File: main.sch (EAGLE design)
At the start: 45 parts, among them IC1 ATTINY13A-SSH, IC2 TP4056-42-ESOP8, IC3 LM27313XMFX_NOPB, IC4 TPL5110DDCT, IC5 ATTINY13A-SSH, T1A 2N4401, T1B NPN, X1 MINI-USB-UX60A-MB-5ST, X2 332-02

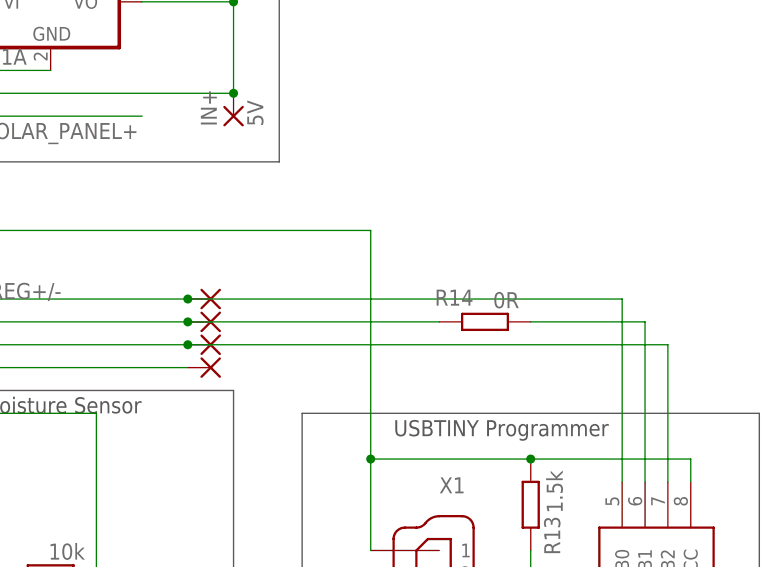
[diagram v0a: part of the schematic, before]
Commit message: updates
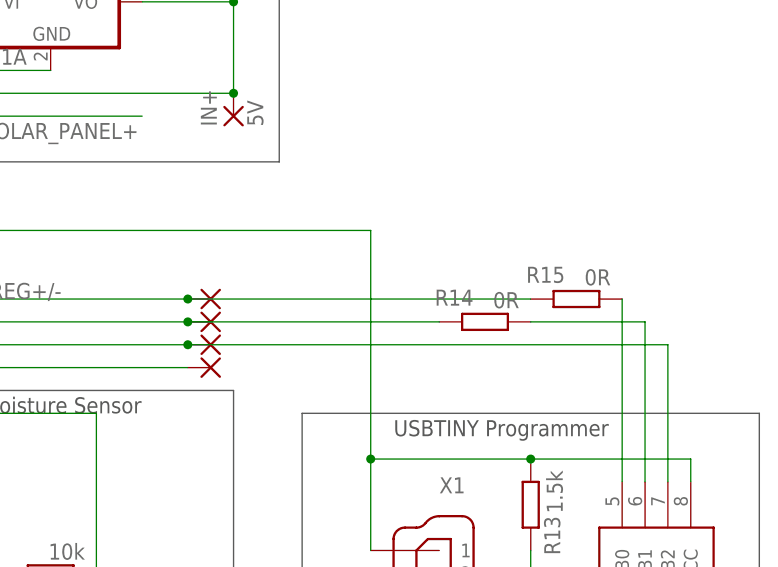
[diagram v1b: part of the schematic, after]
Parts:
- added R15: 0R, resistor:R-EU_R0402
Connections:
- new net N$16: IC5.PB0, R15.1
- net SOLAR_REG+/-: now also R15.2; no longer IC5.PB0
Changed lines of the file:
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@@
 <?xml version="1.0" encoding="utf-8"?>
 <!DOCTYPE eagle SYSTEM "eagle.dtd">
-<eagle version="9.5.2">
+<eagle version="9.6.0">
 <drawing>
 <settings>
@@
 <part name="GND4" library="supply1" library_urn="urn:adsk.eagle:library:371" deviceset="GND" device=""/>
 <part name="R14" library="resistor" library_urn="urn:adsk.eagle:library:348" deviceset="R-EU_" device="R0402" package3d_urn="urn:adsk.eagle:package:26058/1" value="0R"/>
+<part name="R15" library="resistor" library_urn="urn:adsk.eagle:library:348" deviceset="R-EU_" device="R0402" package3d_urn="urn:adsk.eagle:package:26058/1" value="0R"/>
 </parts>
 <sheets>
@@
 <attribute name="VALUE" x="163.83" y="59.182" size="1.778" layer="96" rot="R180"/>
 </instance>
+<instance part="R15" gate="G$1" x="170.18" y="58.42" smashed="yes" rot="R180">
+<attribute name="NAME" x="168.91" y="62.0014" size="1.778" layer="95" rot="R180"/>
+<attribute name="VALUE" x="173.99" y="61.722" size="1.778" layer="96" rot="R180"/>
+</instance>
 </instances>
 <busses>
@@
 <junction x="91.44" y="63.5"/>
 <junction x="91.44" y="58.42"/>
-<pinref part="IC5" gate="G$1" pin="PB0"/>
-<wire x1="175.26" y1="38.1" x2="175.26" y2="58.42" width="0.1524" layer="91"/>
-<wire x1="175.26" y1="58.42" x2="127" y2="58.42" width="0.1524" layer="91"/>
+<pinref part="R15" gate="G$1" pin="2"/>
+<wire x1="165.1" y1="58.42" x2="127" y2="58.42" width="0.1524" layer="91"/>
 <junction x="127" y="58.42"/>
 </segment>
@@
 </segment>
 </net>
+<net name="N$16" class="0">
+<segment>
+<pinref part="IC5" gate="G$1" pin="PB0"/>
+<wire x1="175.26" y1="38.1" x2="175.26" y2="58.42" width="0.1524" layer="91"/>
+<pinref part="R15" gate="G$1" pin="1"/>
+</segment>
+</net>

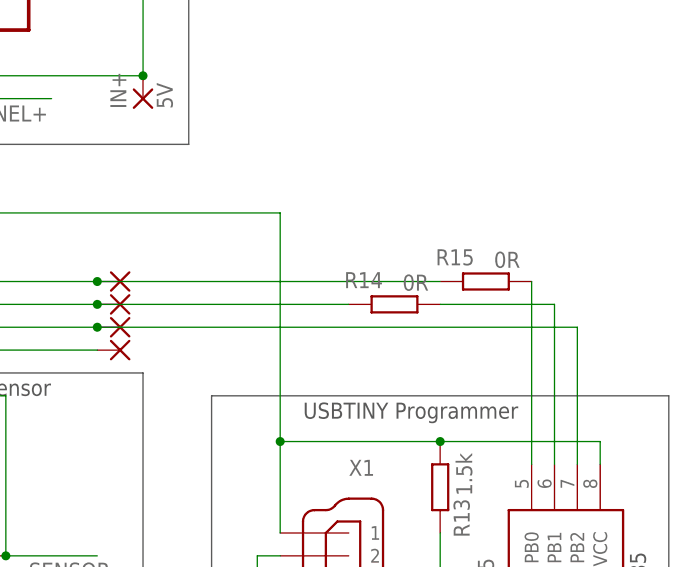
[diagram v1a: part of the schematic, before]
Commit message: updates
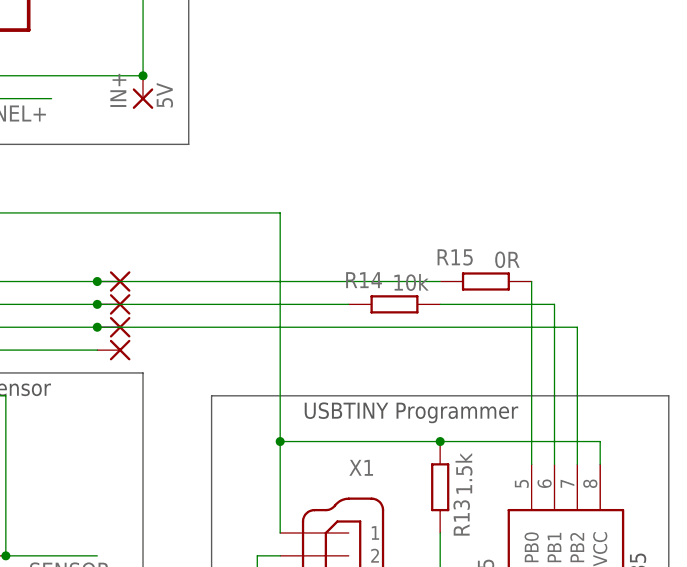
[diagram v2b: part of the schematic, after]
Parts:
- R14: value 0R -> 10k
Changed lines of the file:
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@@
 <part name="R13" library="resistor" library_urn="urn:adsk.eagle:library:348" deviceset="R-EU_" device="R0603" package3d_urn="urn:adsk.eagle:package:23555/2" value="1.5k"/>
 <part name="GND4" library="supply1" library_urn="urn:adsk.eagle:library:371" deviceset="GND" device=""/>
-<part name="R14" library="resistor" library_urn="urn:adsk.eagle:library:348" deviceset="R-EU_" device="R0402" package3d_urn="urn:adsk.eagle:package:26058/1" value="0R"/>
+<part name="R14" library="resistor" library_urn="urn:adsk.eagle:library:348" deviceset="R-EU_" device="R0402" package3d_urn="urn:adsk.eagle:package:26058/1" value="10k"/>
 <part name="R15" library="resistor" library_urn="urn:adsk.eagle:library:348" deviceset="R-EU_" device="R0402" package3d_urn="urn:adsk.eagle:package:26058/1" value="0R"/>
 </parts>
